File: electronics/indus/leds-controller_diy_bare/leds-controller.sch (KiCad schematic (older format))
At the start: 19 parts, among them P1 ALIM_12V_60V, P10 THERM_LEDS, P2 MICRO_CTRL, P3 FANS, P4 POT_COLOR2, P5 POT_COLOR3, P6 POT_COLOR4, P7 POT_COLOR1, P8 LED+, P9 LED-

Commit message: added pin with lock footprint
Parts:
- P10: footprint Connect:PINHEAD1-3 -> risebox:PINHEAD_LOCK_1-3
- P2: footprint risebox:PINHEAD1-10 -> risebox:PINHEAD_LOCK_1-10
- P3: footprint Connect:PINHEAD1-2 -> risebox:PINHEAD_LOCK_1-2
- P8, P9: footprint risebox:PINHEAD1-4 -> risebox:PINHEAD_LOCK_1-4
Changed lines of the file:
@@
 F 0 "P3" H 10800 5700 50  0000 C CNN
 F 1 "FANS" V 10900 5550 50  0000 C CNN
-F 2 "Connect:PINHEAD1-2" H 10800 5550 60  0001 C CNN
+F 2 "risebox:PINHEAD_LOCK_1-2" H 10800 5550 60  0001 C CNN
 F 3 "" H 10800 5550 60  0000 C CNN
 	1    10800 5550
@@
 F 0 "P8" H 10800 2850 50  0000 C CNN
 F 1 "LED+" V 10900 2600 50  0000 C CNN
-F 2 "risebox:PINHEAD1-4" H 10800 2600 50  0001 C CNN
+F 2 "risebox:PINHEAD_LOCK_1-4" H 10800 2600 50  0001 C CNN
 F 3 "" H 10800 2600 50  0000 C CNN
 	1    10800 2600
@@
 F 0 "P9" H 10800 4150 50  0000 C CNN
 F 1 "LED-" V 10900 3900 50  0000 C CNN
-F 2 "risebox:PINHEAD1-4" H 10800 3900 50  0001 C CNN
+F 2 "risebox:PINHEAD_LOCK_1-4" H 10800 3900 50  0001 C CNN
 F 3 "" H 10800 3900 50  0000 C CNN
 	1    10800 3900
@@
 F 0 "P2" H 850 5650 50  0000 C CNN
 F 1 "MICRO_CTRL" V 950 5300 50  0000 C CNN
-F 2 "risebox:PINHEAD1-10" H 850 5300 50  0001 C CNN
+F 2 "risebox:PINHEAD_LOCK_1-10" H 850 5300 50  0001 C CNN
 F 3 "" H 850 5300 50  0000 C CNN
 	1    850  5300
@@
 F 0 "P10" H 850 3950 50  0000 C CNN
 F 1 "THERM_LEDS" V 950 3750 50  0000 C CNN
-F 2 "Connect:PINHEAD1-3" H 850 3750 50  0001 C CNN
+F 2 "risebox:PINHEAD_LOCK_1-3" H 850 3750 50  0001 C CNN
 F 3 "" H 850 3750 50  0000 C CNN
 	1    850  3750

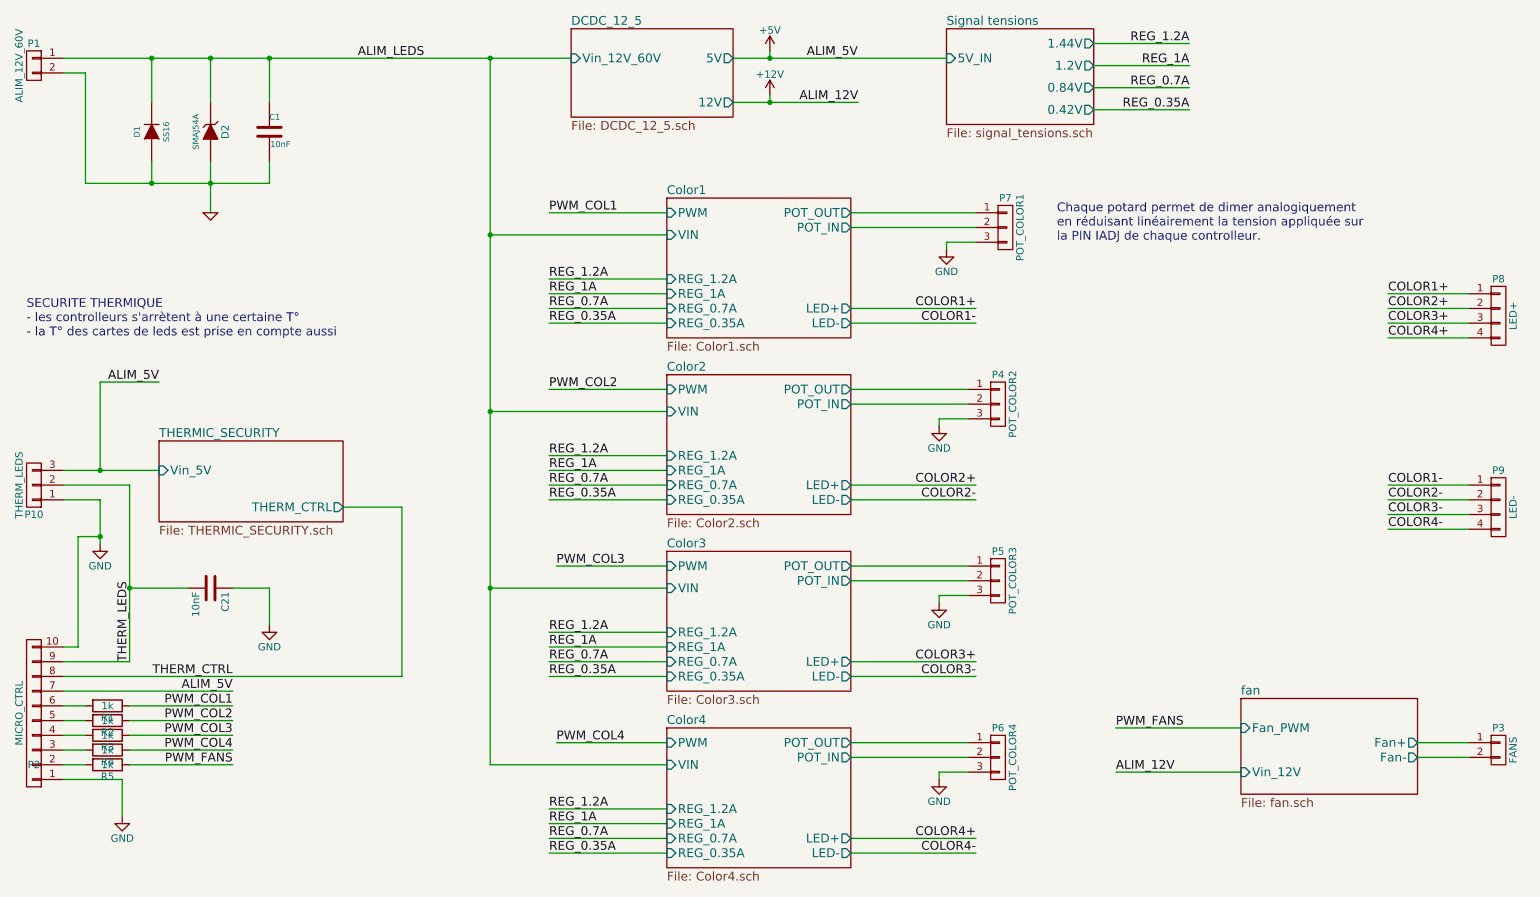
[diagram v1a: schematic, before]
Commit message: led outputs
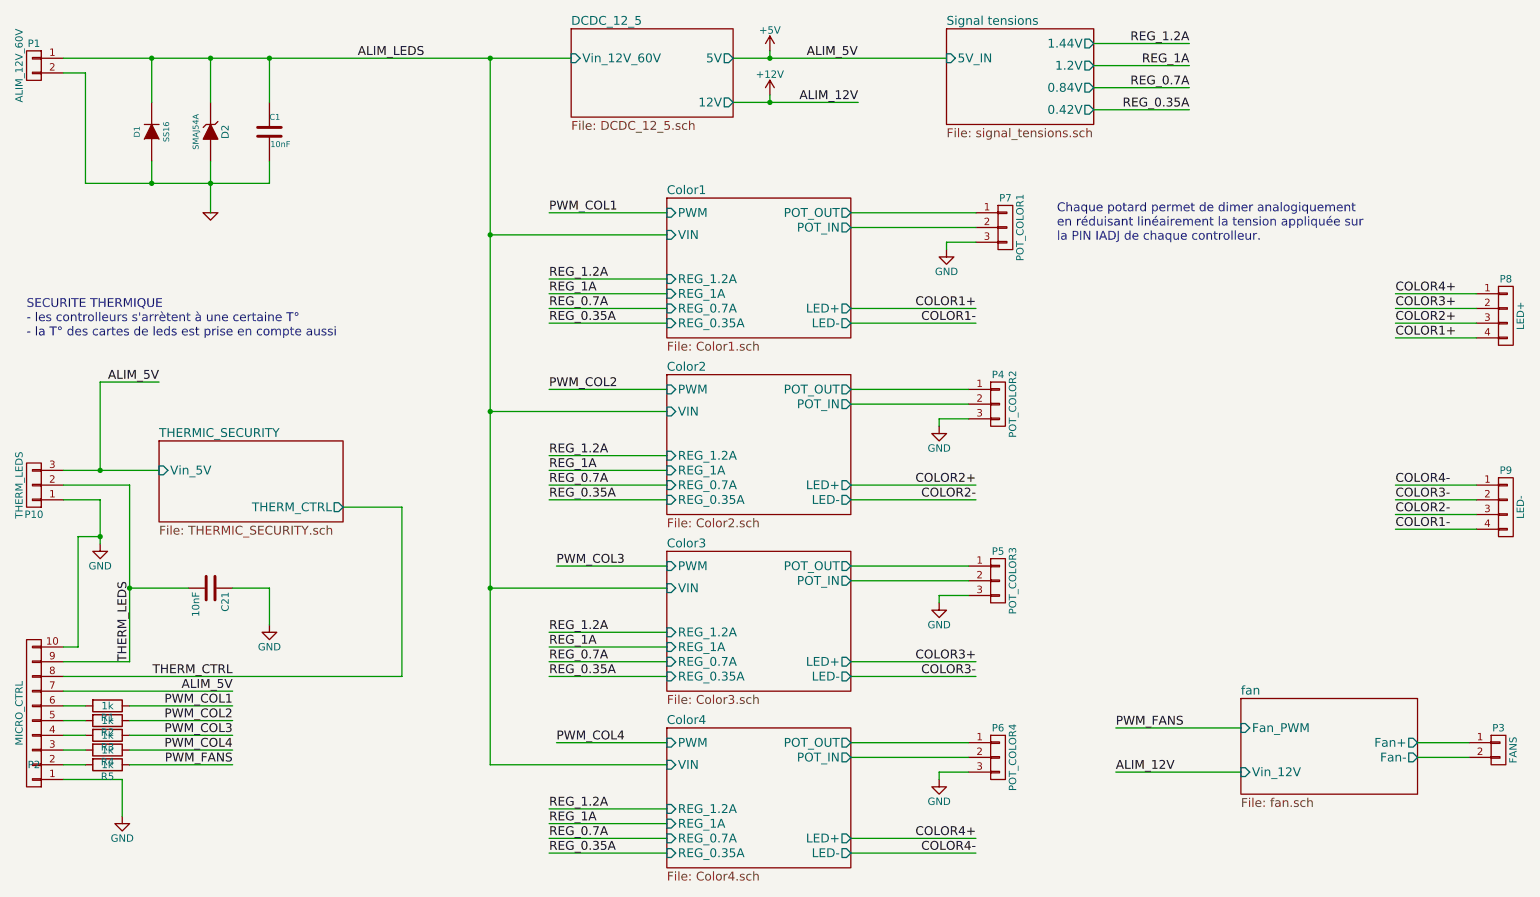
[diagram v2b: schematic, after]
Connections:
- net COLOR1+: now also P8.4 (P4); no longer P8.1 (P1)
- net COLOR1-: now also P9.4 (P4); no longer P9.1 (P1)
- net COLOR2+: now also P8.3 (P3); no longer P8.2 (P2)
- net COLOR2-: now also P9.3 (P3); no longer P9.2 (P2)
- net COLOR3+: now also P8.2 (P2); no longer P8.3 (P3)
- net COLOR3-: now also P9.2 (P2); no longer P9.3 (P3)
- net COLOR4+: now also P8.1 (P1); no longer P8.4 (P4)
- net COLOR4-: now also P9.1 (P1); no longer P9.4 (P4)
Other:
- moved on the sheet: P8, P9
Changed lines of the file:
@@
 L CONN_01X04 P8
 U 1 1 57611EA6
-P 10800 2600
-F 0 "P8" H 10800 2850 50  0000 C CNN
-F 1 "LED+" V 10900 2600 50  0000 C CNN
-F 2 "risebox:PINHEAD_LOCK_1-4" H 10800 2600 50  0001 C CNN
-F 3 "" H 10800 2600 50  0000 C CNN
-	1    10800 2600
+P 10850 2600
+F 0 "P8" H 10850 2850 50  0000 C CNN
+F 1 "LED+" V 10950 2600 50  0000 C CNN
+F 2 "risebox:PINHEAD_LOCK_1-4" H 10850 2600 50  0001 C CNN
+F 3 "" H 10850 2600 50  0000 C CNN
+	1    10850 2600
 	1    0    0    -1
 $EndComp
@@
 L CONN_01X04 P9
 U 1 1 57611FC3
-P 10800 3900
-F 0 "P9" H 10800 4150 50  0000 C CNN
-F 1 "LED-" V 10900 3900 50  0000 C CNN
-F 2 "risebox:PINHEAD_LOCK_1-4" H 10800 3900 50  0001 C CNN
-F 3 "" H 10800 3900 50  0000 C CNN
-	1    10800 3900
+P 10850 3900
+F 0 "P9" H 10850 4150 50  0000 C CNN
+F 1 "LED-" V 10950 3900 50  0000 C CNN
+F 2 "risebox:PINHEAD_LOCK_1-4" H 10850 3900 50  0001 C CNN
+F 3 "" H 10850 3900 50  0000 C CNN
+	1    10850 3900
 	1    0    0    -1
 $EndComp
@@
 Text Label 4350 2650 0    60   ~ 0
 REG_0.35A
-Text Label 10050 2450 0    60   ~ 0
+Text Label 10100 2750 0    60   ~ 0
 COLOR1+
-Text Label 10050 2550 0    60   ~ 0
+Text Label 10100 2650 0    60   ~ 0
 COLOR2+
-Text Label 10050 2650 0    60   ~ 0
+Text Label 10100 2550 0    60   ~ 0
 COLOR3+
-Text Label 10050 2750 0    60   ~ 0
+Text Label 10100 2450 0    60   ~ 0
 COLOR4+
-Text Label 10050 3750 0    60   ~ 0
+Text Label 10100 4050 0    60   ~ 0
 COLOR1-
-Text Label 10050 3850 0    60   ~ 0
+Text Label 10100 3950 0    60   ~ 0
 COLOR2-
-Text Label 10050 3950 0    60   ~ 0
+Text Label 10100 3850 0    60   ~ 0
 COLOR3-
-Text Label 10050 4050 0    60   ~ 0
+Text Label 10100 3750 0    60   ~ 0
 COLOR4-
 $Comp
@@
 	5150 1900 4350 1900
 Wire Wire Line
-	1050 3650 1700 3650
+	1050 3650 1300 3650
+Wire Wire Line
+	1300 3650 1700 3650
 Wire Wire Line
 	5150 2050 3950 2050
 Connection ~ 3950 850
 Wire Wire Line
-	1300 3850 1300 4150
+	1300 3850 1300 4100
+Wire Wire Line
+	1300 4100 1300 4150
 Wire Wire Line
 	1050 3850 1300 3850
 Wire Wire Line
-	5600 1150 6450 1150
-Wire Wire Line
-	5600 850  7050 850
+	5600 1150 5850 1150
+Wire Wire Line
+	5850 1150 6450 1150
+Wire Wire Line
+	5600 850  5850 850
+Wire Wire Line
+	5850 850  7050 850
 Wire Wire Line
 	1450 5750 1450 6000
@@
 	1650 1550 1650 1700
 Wire Wire Line
-	2050 1550 2050 1900
-Wire Wire Line
-	1200 1700 2450 1700
+	2050 1550 2050 1700
+Wire Wire Line
+	2050 1700 2050 1900
+Wire Wire Line
+	1200 1700 1650 1700
+Wire Wire Line
+	1650 1700 2050 1700
+Wire Wire Line
+	2050 1700 2450 1700
 Connection ~ 2450 850
 Wire Wire Line
@@
 	6400 3100 7200 3100
 Wire Wire Line
-	10600 4050 10050 4050
-Wire Wire Line
-	10600 3950 10050 3950
-Wire Wire Line
-	10600 3850 10050 3850
-Wire Wire Line
-	10600 3750 10050 3750
-Wire Wire Line
-	10600 2750 10050 2750
-Wire Wire Line
-	10600 2650 10050 2650
-Wire Wire Line
-	10600 2550 10050 2550
-Wire Wire Line
-	10600 2450 10050 2450
+	10650 3750 10100 3750
+Wire Wire Line
+	10650 3850 10100 3850
+Wire Wire Line
+	10650 3950 10100 3950
+Wire Wire Line
+	10650 4050 10100 4050
+Wire Wire Line
+	10650 2450 10100 2450
+Wire Wire Line
+	10650 2550 10100 2550
+Wire Wire Line
+	10650 2650 10100 2650
+Wire Wire Line
+	10650 2750 10100 2750
 Wire Wire Line
 	6400 2650 7250 2650
@@
 	3950 5650 5150 5650
 Wire Wire Line
-	3950 850  3950 5650
+	3950 850  3950 2050
+Wire Wire Line
+	3950 2050 3950 3250
+Wire Wire Line
+	3950 3250 3950 4450
+Wire Wire Line
+	3950 4450 3950 5650
 Wire Wire Line
 	10250 5500 10600 5500
@@
 	8200 5700 9050 5700
 Wire Wire Line
-	1050 850  4500 850
+	1050 850  1650 850
+Wire Wire Line
+	1650 850  2050 850
+Wire Wire Line
+	2050 850  2450 850
+Wire Wire Line
+	2450 850  3950 850
+Wire Wire Line
+	3950 850  4500 850
 Wire Wire Line
 	1200 950  1200 1700
@@
 	3350 5050 1050 5050
 Wire Wire Line
-	1500 3750 1500 4950
+	1500 3750 1500 4450
+Wire Wire Line
+	1500 4450 1500 4950
 Wire Wire Line
 	1500 4950 1050 4950

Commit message: something...
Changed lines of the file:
@@
 	5150 1900 4350 1900
 Wire Wire Line
-	1050 3650 1300 3650
-Wire Wire Line
-	1300 3650 1700 3650
+	1050 3650 1700 3650
 Wire Wire Line
 	5150 2050 3950 2050
 Connection ~ 3950 850
 Wire Wire Line
-	1300 3850 1300 4100
-Wire Wire Line
-	1300 4100 1300 4150
+	1300 3850 1300 4150
 Wire Wire Line
 	1050 3850 1300 3850
 Wire Wire Line
-	5600 1150 5850 1150
+	5600 1150 6450 1150
 Wire Wire Line
-	5850 1150 6450 1150
-Wire Wire Line
-	5600 850  5850 850
-Wire Wire Line
-	5850 850  7050 850
+	5600 850  7050 850
 Wire Wire Line
 	1450 5750 1450 6000
@@
 	1650 1550 1650 1700
 Wire Wire Line
-	2050 1550 2050 1700
+	2050 1550 2050 1900
 Wire Wire Line
-	2050 1700 2050 1900
-Wire Wire Line
-	1200 1700 1650 1700
-Wire Wire Line
-	1650 1700 2050 1700
-Wire Wire Line
-	2050 1700 2450 1700
+	1200 1700 2450 1700
 Connection ~ 2450 850
 Wire Wire Line
@@
 	3950 5650 5150 5650
 Wire Wire Line
-	3950 850  3950 2050
-Wire Wire Line
-	3950 2050 3950 3250
-Wire Wire Line
-	3950 3250 3950 4450
-Wire Wire Line
-	3950 4450 3950 5650
+	3950 850  3950 5650
 Wire Wire Line
 	10250 5500 10600 5500
@@
 	8200 5700 9050 5700
 Wire Wire Line
-	1050 850  1650 850
-Wire Wire Line
-	1650 850  2050 850
-Wire Wire Line
-	2050 850  2450 850
-Wire Wire Line
-	2450 850  3950 850
-Wire Wire Line
-	3950 850  4500 850
+	1050 850  4500 850
 Wire Wire Line
 	1200 950  1200 1700
@@
 	3350 5050 1050 5050
 Wire Wire Line
-	1500 3750 1500 4450
-Wire Wire Line
-	1500 4450 1500 4950
+	1500 3750 1500 4950
 Wire Wire Line
 	1500 4950 1050 4950
